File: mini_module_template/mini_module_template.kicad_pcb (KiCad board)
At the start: 4 copper layers, 100 x 50 mm, 135 parts, among them IC1 TJA1044GTK_3Z, J1 SWD, J4 USB_C_Receptacle_USB2.0, Q1 S9013, SW2 NRST, SW4 SW_DIP_x01, U1 STM32F303CBTx, U2 FM24CL16B, U3 STM32F103CB, U4 AZ1117-3.3, U5 TPS563200, U6 IP4220CZ6, U7 SL2.1A, Y1 8MHz, Y2 8MHz, Y4 12Mhz

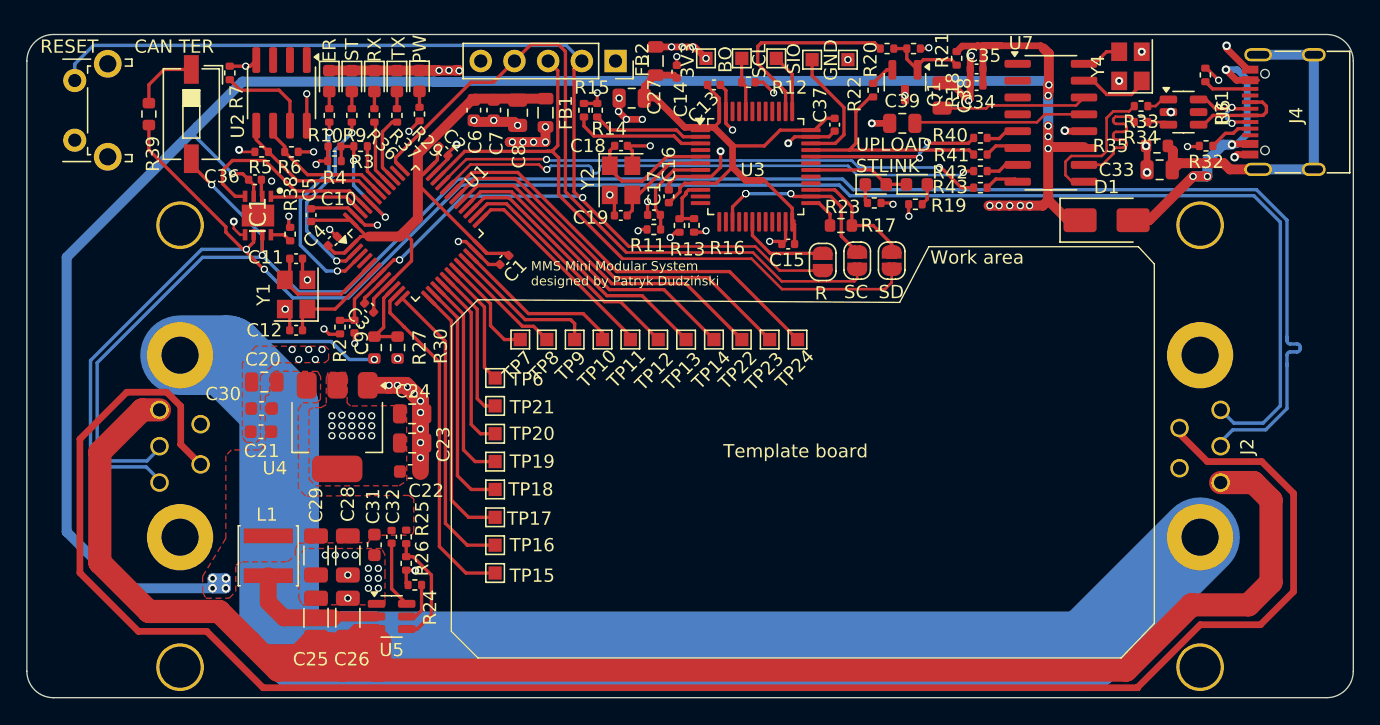
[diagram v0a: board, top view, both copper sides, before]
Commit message: a
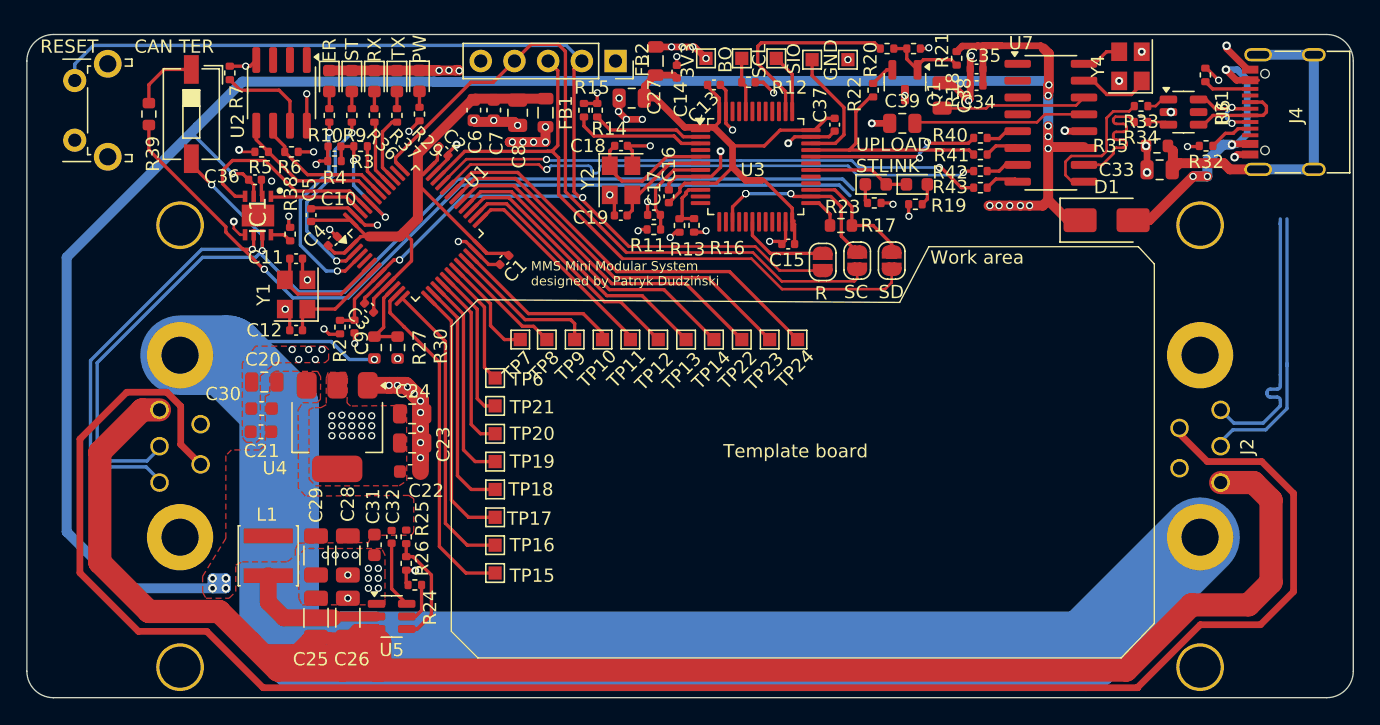
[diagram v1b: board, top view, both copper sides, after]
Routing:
- net /CAN/CANH: track 144.6 -> 109.2 mm
- net /CAN/CANL: track 146.0 -> 115.4 mm
